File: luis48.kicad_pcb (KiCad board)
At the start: 2 copper layers, 127 x 110 mm, 3 parts, among them M1 Module-ign8-0.2, U1 ISL9V3040D3ST-F085C, U2 5007620481

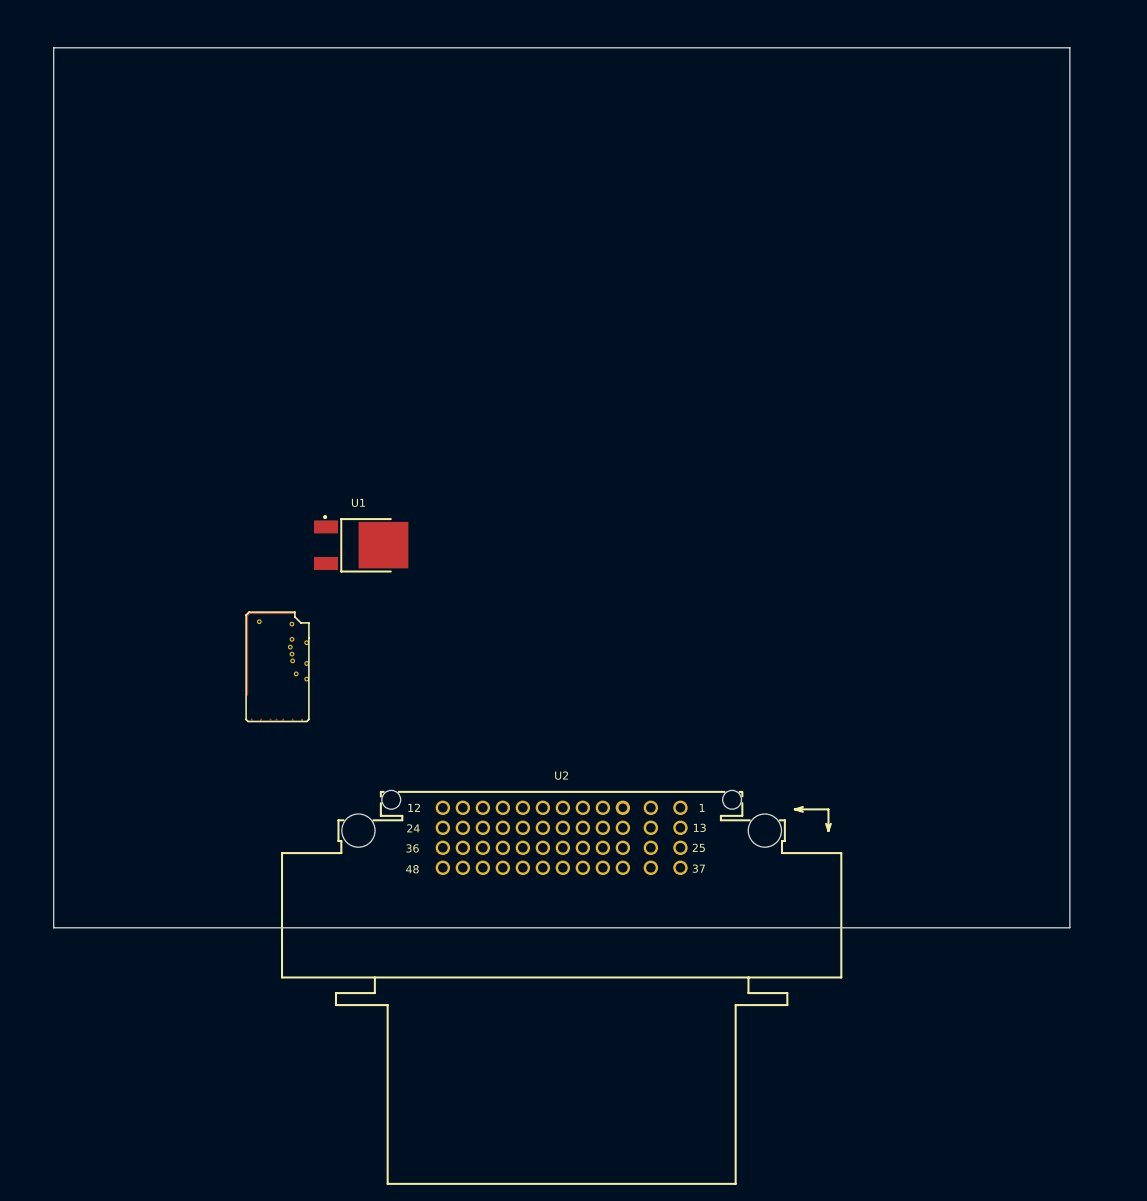
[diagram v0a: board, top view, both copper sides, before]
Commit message: wew
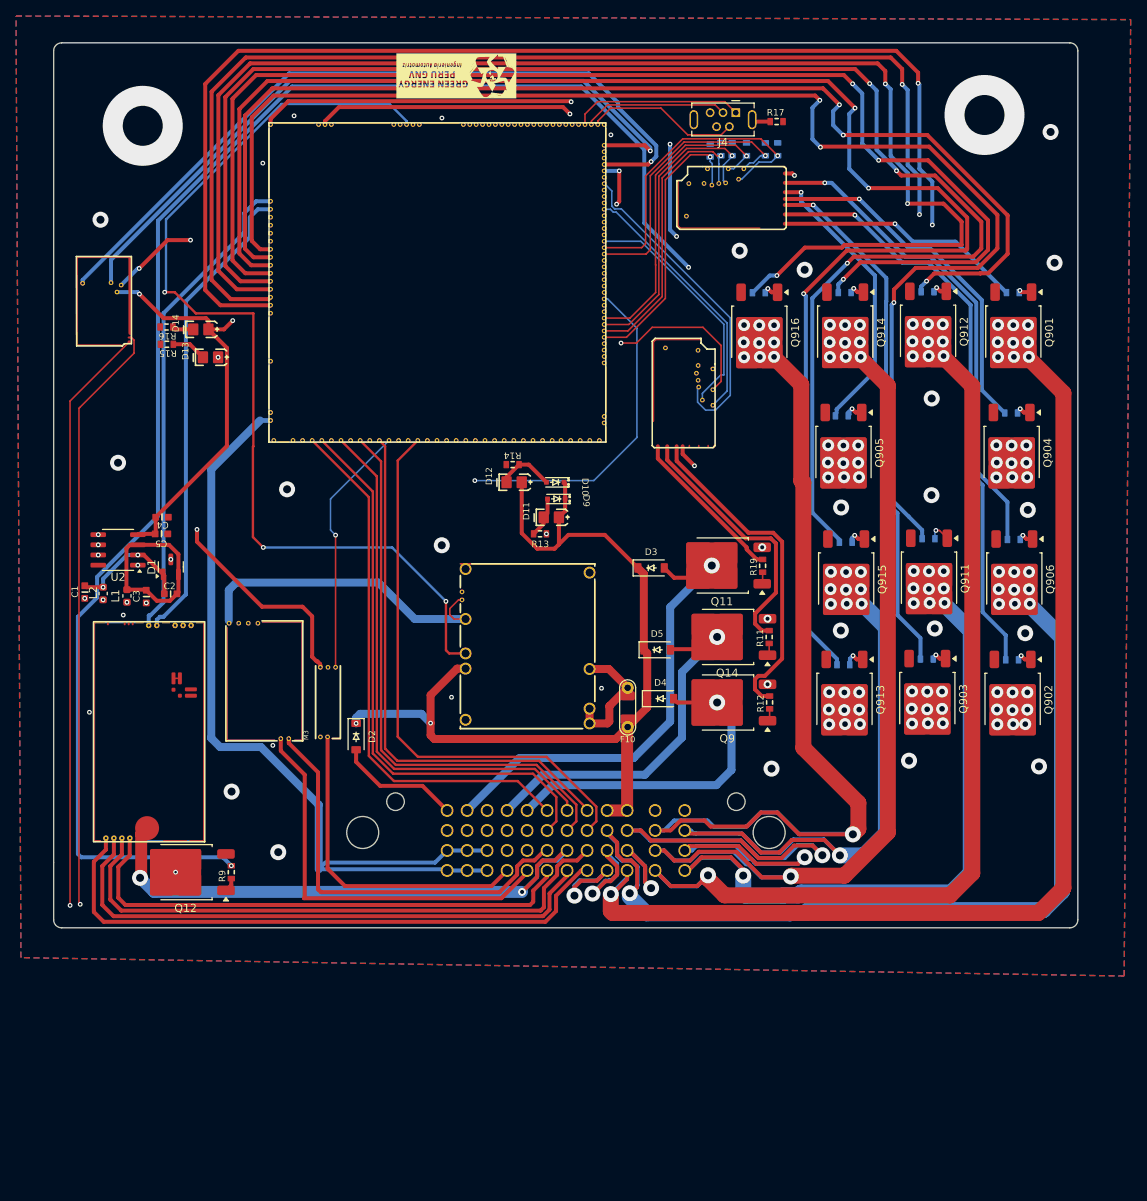
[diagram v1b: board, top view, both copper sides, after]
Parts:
- added C1: 10n, hellen-one-common:C0603, F.Cu at (53.4, 57.5)
- added C2: 100n, hellen-one-common:C0603, F.Cu at (64.1, 57.7)
- added C3: 10n, hellen-one-common:C0603, F.Cu at (61.1, 58.1)
- added C4: 100n, hellen-one-common:C0603, F.Cu at (63.0, 48.2)
- added C5: 1u, hellen-one-common:C0603, F.Cu at (63.0, 50.3)
- added D1: NUP2105L, Package_TO_SOT_SMD:SOT-23, F.Cu at (64.1, 54.4)
- added D10: 1N4148WS, hellen-one-common:SOD-323, F.Cu at (112.2, 43.8)
- added D11: LED-GREEN-0805, hellen-one-common:LED-0805, F.Cu at (111.7, 48.2)
- added D12: LED-GREEN-0805, hellen-one-common:LED-0805, F.Cu at (107.1, 43.8)
- added D13: LED-GREEN-0805, hellen-one-common:LED-0805, F.Cu at (69.1, 28.2)
- added D14: LED-GREEN-0805, hellen-one-common:LED-0805, F.Cu at (67.9, 24.7)
- added D2: B5819W, hellen-one-common:SOD-123, F.Cu at (87.3, 75.6)
- added D3: B5819W, hellen-one-common:SOD-123, F.Cu at (124.2, 54.5)
- added D4: B5819W, hellen-one-common:SOD-123, F.Cu at (125.3, 70.9)
- added D5: B5819W, hellen-one-common:SOD-123, F.Cu at (124.9, 64.8)
- added D9: 1N4148WS, hellen-one-common:SOD-323, F.Cu at (112.3, 45.9)
- added F10: Fuse-Pad-Pad, hellen-one-common:PAD-1206-PAD, F.Cu at (121.2, 72.0)
- added G***: LOGO, GDI-6ch:lokone, F.Cu at (99.8, -6.97)
- added G***: LOGO, GDI-6ch:lokone, B.Cu at (99.8, -6.99)
- added J4: USB_B_Mini, hellen-one-common:USB-MINI-B-VERTICAL, F.Cu at (133.2, -1.52)
- added L1: 470R@100MHz, Inductor_SMD:L_0603_1608Metric, F.Cu at (58.7, 58.0)
- added L2: 470R@100MHz, Inductor_SMD:L_0603_1608Metric, F.Cu at (55.7, 57.7)
- added M3: Module-knock-0.2, knock-0.2:knock, F.Cu at (85.4, 75.9)
- added M4: Module-ign8-0.2, ign8-0.2:ign8, F.Cu at (141.2, 12.2)
- added M5: Module-wbo-0.5, wbo-0.5:wbo, F.Cu at (54.4, 61.1)
- added M6: Module-can-0.1, can-01:can, F.Cu at (59.3, 26.9)
- added M7: Module-ign8-0.2, ign8-0.2:ign8, F.Cu at (124.3, 39.6)
- added M8: Module-vr-max9924-0.1, vr-max9924-0.1:vr-max9924, F.Cu at (80.7, 76.2)
- added M9: Module-mega-mcu144-0.7, mega-144-07:mega-mcu144, F.Cu at (76.3, 38.9)
- added Q11: ISL9V3040D3ST, Package_TO_SOT_SMD:TO-252-2, F.Cu at (133.0, 54.2)
- added Q12: ISL9V3040D3ST, Package_TO_SOT_SMD:TO-252-2, F.Cu at (66.0, 92.5)
- added Q14: ISL9V3040D3ST, Package_TO_SOT_SMD:TO-252-2, F.Cu at (133.7, 63.1)
- added Q9: ISL9V3040D3ST, Package_TO_SOT_SMD:TO-252-2, F.Cu at (133.7, 71.3)
- added Q901: ISL9V3040D3ST, Package_TO_SOT_SMD:TO-252-2, F.Cu at (169.5, 25.1)
- added Q902: ISL9V3040D3ST, Package_TO_SOT_SMD:TO-252-2, F.Cu at (169.4, 71.0)
- added Q903: ISL9V3040D3ST, Package_TO_SOT_SMD:TO-252-2, F.Cu at (158.7, 70.9)
- added Q904: ISL9V3040D3ST, Package_TO_SOT_SMD:TO-252-2, F.Cu at (169.2, 40.1)
- added Q905: ISL9V3040D3ST, Package_TO_SOT_SMD:TO-252-2, F.Cu at (148.2, 40.1)
- added Q906: ISL9V3040D3ST, Package_TO_SOT_SMD:TO-252-2, F.Cu at (169.6, 55.9)
- added Q911: ISL9V3040D3ST, Package_TO_SOT_SMD:TO-252-2, F.Cu at (158.9, 55.8)
- added Q912: ISL9V3040D3ST, Package_TO_SOT_SMD:TO-252-2, F.Cu at (158.8, 25.0)
- added Q913: ISL9V3040D3ST, Package_TO_SOT_SMD:TO-252-2, F.Cu at (148.3, 71.0)
- added Q914: ISL9V3040D3ST, Package_TO_SOT_SMD:TO-252-2, F.Cu at (148.4, 25.1)
- added Q915: ISL9V3040D3ST, Package_TO_SOT_SMD:TO-252-2, F.Cu at (148.6, 55.9)
- added Q916: ISL9V3040D3ST, Package_TO_SOT_SMD:TO-252-2, F.Cu at (137.7, 25.1)
- added R11: 22, hellen-one-common:R0603, F.Cu at (138.9, 63.2)
- added R12: 22, hellen-one-common:R0603, F.Cu at (139.0, 71.3)
- added R13: 5.1k, hellen-one-common:R0603, F.Cu at (110.3, 50.3)
- added R14: 5.1k, hellen-one-common:R0603, F.Cu at (106.9, 41.6)
- added R15: 1.6k, hellen-one-common:R0603, F.Cu at (63.7, 26.6)
- added R16: 750, hellen-one-common:R0603, F.Cu at (63.6, 24.4)
- added R17: 0, hellen-one-common:R0603, F.Cu at (139.9, -1.27)
- added R19: 22, hellen-one-common:R0603, F.Cu at (138.1, 54.3)
- added R401: 10k, hellen-one-common:R0603, B.Cu at (138.5, 2.19)
- added R402: 10k, hellen-one-common:R0603, B.Cu at (140.0, 2.19)
- added R403: 10k, hellen-one-common:R0603, B.Cu at (136.1, 2.19)
- added R404: 10k, hellen-one-common:R0603, B.Cu at (134.3, 2.19)
- added R405: 10k, hellen-one-common:R0603, B.Cu at (132.9, 2.19)
- added R406: 10k, hellen-one-common:R0603, B.Cu at (131.6, 2.34)
- added R9: 22, hellen-one-common:R0603, F.Cu at (71.7, 92.5)
- added R901: 22, hellen-one-common:R0603, B.Cu at (169.4, 20.1)
- added R902: 22, hellen-one-common:R0603, B.Cu at (169.3, 66.0)
- added R903: 22, hellen-one-common:R0603, B.Cu at (158.7, 65.9)
- added R904: 22, hellen-one-common:R0603, B.Cu at (169.2, 35.1)
- added R905: 22, hellen-one-common:R0603, B.Cu at (148.0, 35.5)
- added R906: 22, hellen-one-common:R0603, B.Cu at (169.5, 51.0)
- added R911: 22, hellen-one-common:R0603, B.Cu at (158.9, 50.9)
- added R912: 22, hellen-one-common:R0603, B.Cu at (158.7, 20.0)
- added R913: 22, hellen-one-common:R0603, B.Cu at (148.2, 66.6)
- added R914: 22, hellen-one-common:R0603, B.Cu at (148.4, 20.1)
- added R915: 22, hellen-one-common:R0603, B.Cu at (148.5, 51.3)
- added R916: 22, hellen-one-common:R0603, B.Cu at (137.7, 20.1)
- M1: value Module-ign8-0.2 -> Module-power_12and5V-0.1; footprint hellen-one-ign8-0.2:ign8 -> power-12-5v-0.1:power_12and5V
- U1: value ISL9V3040D3ST-F085C -> molex_48pin_MRE; footprint jlc_footprints:JLC_DPAK_L6.5-W6.0-P2.29-LS9.9-TL -> conector-mre48:Molex_48_MRE
- U2: value 5007620481 -> MAX31855KASA; footprint jlc_footprints:CONN-TH_5007620481 -> Package_SO:SOIC-8_3.9x4.9mm_P1.27mm
- moved U2 66.1 mm to (57.5, 52.3), turned to 180 degrees
- moved U1 57.9 mm to (128.4, 92.3), turned to 180 degrees
- moved M1 48.0 mm to (117.2, 53.9), turned to 180 degrees
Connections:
- M1 pad S1: unconnected-(M1-OUT_IGN8-PadS1) -> (no net)
- M1 pad V1: unconnected-(M1-IGN8-PadV1) -> (no net)
- M1 pad V2: unconnected-(M1-IGN7-PadV2) -> (no net)
- M1 pad V3: unconnected-(M1-IGN6-PadV3) -> (no net)
- M1 pad V4: unconnected-(M1-IGN5-PadV4) -> (no net)
- U1 pad 1: unconnected-(U1-G-Pad1) -> (no net)
- U1 pad 3: unconnected-(U1-E-Pad3) -> (no net)
- U1 pad 4: unconnected-(U1-C-Pad4) -> (no net)
- U2 pad 1: unconnected-(U2-Pad1) -> (no net)
- U2 pad 2: unconnected-(U2-Pad2) -> (no net)
- U2 pad 3: unconnected-(U2-Pad3) -> (no net)
- U2 pad 4: unconnected-(U2-Pad4) -> (no net)
- U2 pad 5: unconnected-(U2-Pad5) -> (no net)
- U2 pad 6: unconnected-(U2-Pad6) -> (no net)
- U2 pad 7: unconnected-(U2-Pad7) -> (no net)
- U2 pad 8: unconnected-(U2-Pad8) -> (no net)
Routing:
- net (no net): track 0.00 -> 5815.9 mm, vias 0 -> 246
- added copper zone on B.Cu, net (none)
- added copper zone on F.Cu, net (none)
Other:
- board size 127 x 110 mm -> 128 x 110.6 mm

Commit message: wew
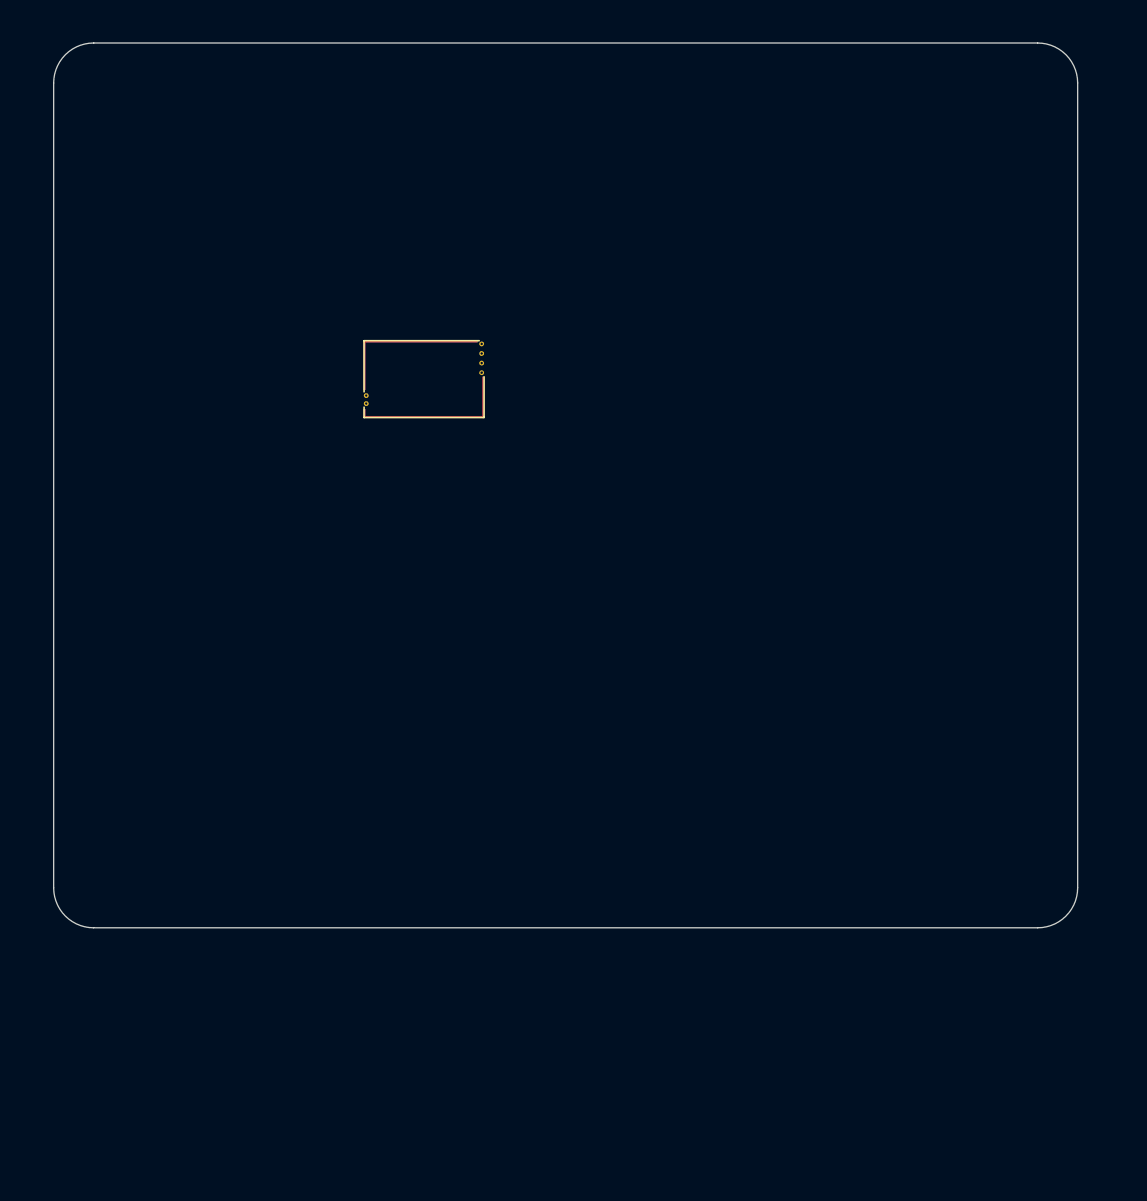
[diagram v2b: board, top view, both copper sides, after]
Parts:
- removed C1, C3: 10n, hellen-one-common:C0603
- removed C2, C4: 100n, hellen-one-common:C0603
- removed C5: 1u, hellen-one-common:C0603
- removed D1: NUP2105L, Package_TO_SOT_SMD:SOT-23
- removed D10, D9: 1N4148WS, hellen-one-common:SOD-323
- removed D11, D12, D13, D14: LED-GREEN-0805, hellen-one-common:LED-0805
- removed D2, D3, D4, D5: B5819W, hellen-one-common:SOD-123
- removed F10: Fuse-Pad-Pad, hellen-one-common:PAD-1206-PAD
- removed G*** (x2): LOGO, GDI-6ch:lokone
- removed J4: USB_B_Mini, hellen-one-common:USB-MINI-B-VERTICAL
- removed L1, L2: 470R@100MHz, Inductor_SMD:L_0603_1608Metric
- removed M3: Module-knock-0.2, knock-0.2:knock
- removed M4, M7: Module-ign8-0.2, ign8-0.2:ign8
- removed M5: Module-wbo-0.5, wbo-0.5:wbo
- removed M6: Module-can-0.1, can-01:can
- removed M8: Module-vr-max9924-0.1, vr-max9924-0.1:vr-max9924
- removed M9: Module-mega-mcu144-0.7, mega-144-07:mega-mcu144
- removed Q11, Q12, Q14, Q9, Q901, Q902, Q903, Q904, Q905, Q906, Q911, Q912, Q913, Q914, Q915, Q916: ISL9V3040D3ST, Package_TO_SOT_SMD:TO-252-2
- removed R11, R12, R19, R9, R901, R902, R903, R904, R905, R906, R911, R912, R913, R914, R915, R916: 22, hellen-one-common:R0603
- removed R13, R14: 5.1k, hellen-one-common:R0603
- removed R15: 1.6k, hellen-one-common:R0603
- removed R16: 750, hellen-one-common:R0603
- removed R17: 0, hellen-one-common:R0603
- removed R401, R402, R403, R404, R405, R406: 10k, hellen-one-common:R0603
- removed U1: molex_48pin_MRE, conector-mre48:Molex_48_MRE
- removed U2: MAX31855KASA, Package_SO:SOIC-8_3.9x4.9mm_P1.27mm
- M1: value Module-power_12and5V-0.1 -> Module-vr-max9924-0.1; footprint power-12-5v-0.1:power_12and5V -> hellen-one-vr-max9924-0.1:vr-max9924
- moved M1 34.2 mm to (88.2, 35.8), turned to 0 degrees
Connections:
- M1 pad E1: (no net) -> unconnected-(M1-NC-PadE1)
- M1 pad E2: (no net) -> unconnected-(M1-NC-PadE2)
- M1 pad E3: (no net) -> unconnected-(M1-OUT-PadE3)
- M1 pad E4: (no net) -> unconnected-(M1-V5_IN-PadE4)
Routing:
- net (no net): track 5815.9 -> 0.00 mm, vias 246 -> 0
- removed copper zone on B.Cu, net (none)
- removed copper zone on F.Cu, net (none)
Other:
- outline, holes or cut-outs redrawn
